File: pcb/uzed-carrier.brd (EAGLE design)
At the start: 100 x 80 mm, 11 parts

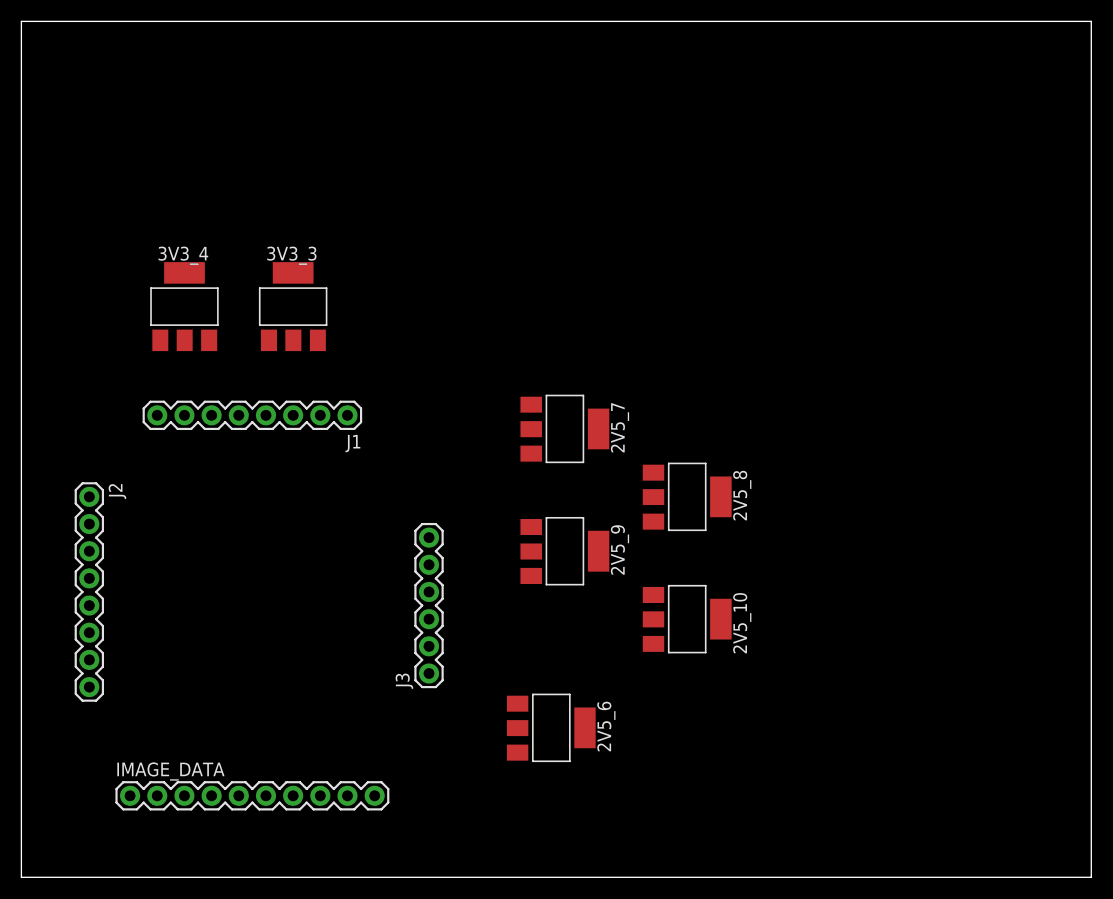
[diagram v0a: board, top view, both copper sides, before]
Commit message: finished with uZed carrier board.
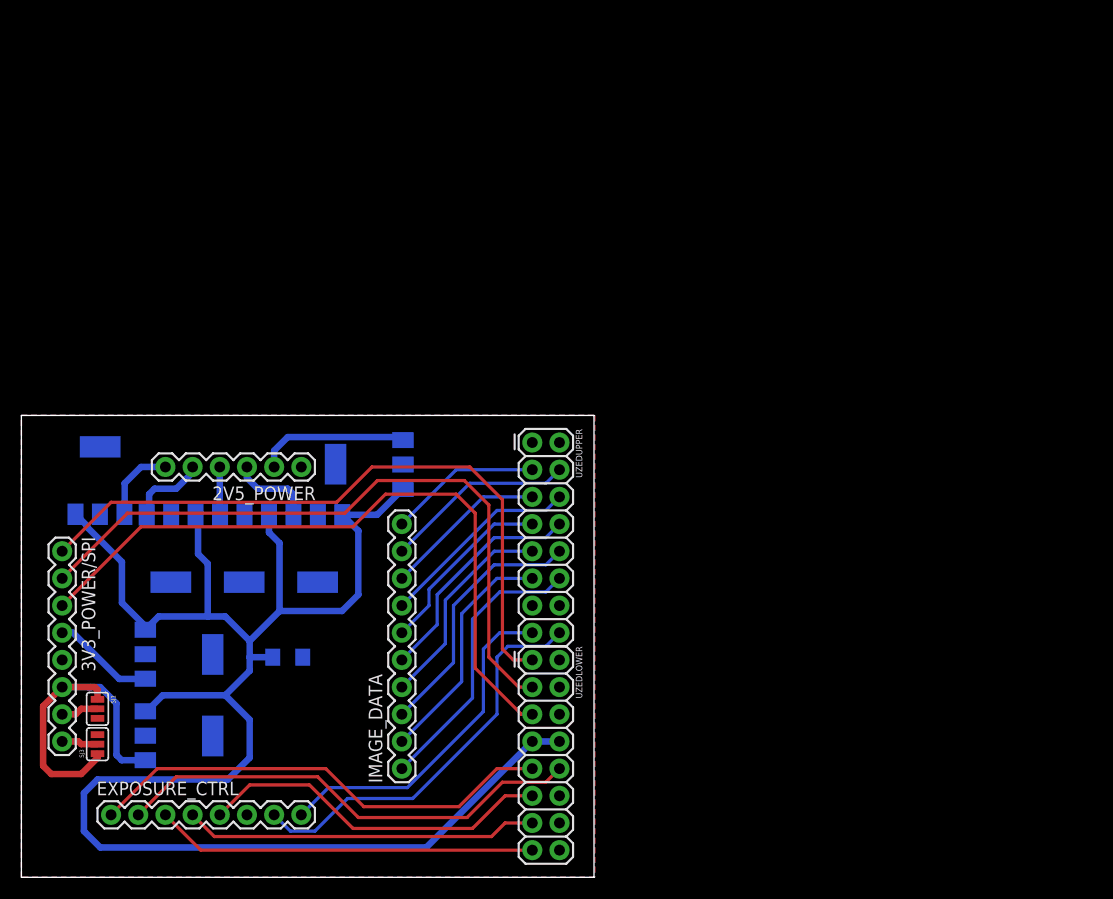
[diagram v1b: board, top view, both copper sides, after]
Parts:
- removed J1, J2: (no value), SparkFun-Connectors:1X08_ROUND
- removed J3: (no value), SparkFun-Connectors:1X06
- added 2V5_POWER: (no value), SparkFun-Connectors:1X06
- added 3V3_POWER/SPI, EXPOSURE_CTRL: (no value), SparkFun-Connectors:1X08_ROUND
- added C1: 10uF, SparkFun-Capacitors:EIA3216
- added SJ1, SJ3: (no value), SparkFun-Retired:SJ_3
- added UZEDLOWER, UZEDUPPER: (no value), SparkFun-Connectors:2X8
- moved 2V5_6 48.1 mm to (7.37, 37.1), flipped to the bottom, turned to 0 degrees
- moved 2V5_8 41.7 mm to (20.8, 30.7), flipped to the bottom, turned to 180 degrees
- moved 3V3_4 40.1 mm to (14.7, 13.2), flipped to the bottom, turned to 90 degrees
- moved 2V5_7 38.5 mm to (14.0, 30.7), flipped to the bottom, turned to 180 degrees
- moved 3V3_3 34.2 mm to (14.7, 20.8), flipped to the bottom, turned to 90 degrees
- moved 2V5_10 33.1 mm to (32.5, 38.6), flipped to the bottom
- moved IMAGE_DATA 25.5 mm to (35.6, 10.2), turned to 90 degrees
- moved 2V5_9 23.1 mm to (27.7, 30.7), flipped to the bottom, turned to 180 degrees
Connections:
- net CLK: now also EXPOSURE_CTRL.8, UZEDUPPER.15; no longer J2.8
- net D0: now also UZEDUPPER.12
- net D1: now also UZEDUPPER.11
- net D2: now also UZEDUPPER.10
- net D3: now also UZEDUPPER.9
- net D4: now also UZEDUPPER.8
- net D5: now also UZEDUPPER.7
- net D6: now also UZEDUPPER.6
- net D7: now also UZEDUPPER.5
- net D8: now also UZEDUPPER.4
- net D9: now also UZEDUPPER.3
- net FRAME_VALID: now also EXPOSURE_CTRL.2, UZEDLOWER.10; no longer J2.2
- net GND: now also 2V5_POWER.1, 3V3_POWER/SPI.5, C1.-, EXPOSURE_CTRL.6, SJ1.3, SJ3.3, UZEDUPPER.1, UZEDUPPER.2; no longer J1.5, J2.6, J3.1
- net INT_TIME1: now also EXPOSURE_CTRL.5, UZEDLOWER.11; no longer J2.5
- net INT_TIME2: now also EXPOSURE_CTRL.4, UZEDLOWER.13; no longer J2.4
- net INT_TIME3: now also EXPOSURE_CTRL.3, UZEDLOWER.15; no longer J2.3
- net LINE_VALID: now also EXPOSURE_CTRL.1, UZEDLOWER.9; no longer J2.1
- net RESET: now also EXPOSURE_CTRL.7, UZEDUPPER.16; no longer J2.7
- net SPI_CLK: now also 3V3_POWER/SPI.2, UZEDLOWER.3; no longer J1.2
- net SPI_DATA: now also 3V3_POWER/SPI.3, UZEDLOWER.5; no longer J1.3
- net SPI_EN: now also 3V3_POWER/SPI.1, UZEDLOWER.1; no longer J1.1
- net VADC: now also 2V5_POWER.4; no longer J3.4
- net VDDA: now also 2V5_POWER.5; no longer J3.5
- net VDDD: now also 2V5_POWER.3; no longer J3.3
- net VDDO: now also 2V5_POWER.2; no longer J3.2
- net VIN: now also C1.+, UZEDLOWER.7, UZEDLOWER.8
- net VMEM_H: now also 3V3_POWER/SPI.4; no longer J1.4
- net VPIX: now also 2V5_POWER.6; no longer J3.6
- net VRESET_1: now also 3V3_POWER/SPI.6, SJ1.1, SJ3.1; no longer J1.6
- net VRESET_2: now also 3V3_POWER/SPI.7, SJ1.2; no longer J1.7
- net VRESET_3: now also 3V3_POWER/SPI.8, SJ3.2; no longer J1.8
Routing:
- net VIN: track 0.00 -> 163.4 mm
- net SPI_DATA: track 0.00 -> 65.3 mm
- net SPI_CLK: track 0.00 -> 64.1 mm
- net SPI_EN: track 0.00 -> 62.9 mm
- net FRAME_VALID: track 0.00 -> 44.3 mm
- net LINE_VALID: track 0.00 -> 44.1 mm
- net RESET: track 0.00 -> 38.1 mm
- net INT_TIME3: track 0.00 -> 35.7 mm
- net INT_TIME1: track 0.00 -> 33.3 mm
- net INT_TIME2: track 0.00 -> 33.1 mm
- net VRESET_1: track 0.00 -> 32.3 mm
- net CLK: track 0.00 -> 32.1 mm
- net D0: track 0.00 -> 26.4 mm
- net D2: track 0.00 -> 24.2 mm
- net D1: track 0.00 -> 22.2 mm
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- added copper zone on layer 1, net GND
- added copper zone on layer 16, net GND
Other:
- board size 100 x 80 mm -> 53.5 x 43.2 mm
- board text added: "LUPA300 + uZED Matt Ruffner 2017 v1.0"
